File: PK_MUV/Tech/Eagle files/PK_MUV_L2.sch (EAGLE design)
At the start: 6 parts, among them U1 WS2812, U2 WS2812

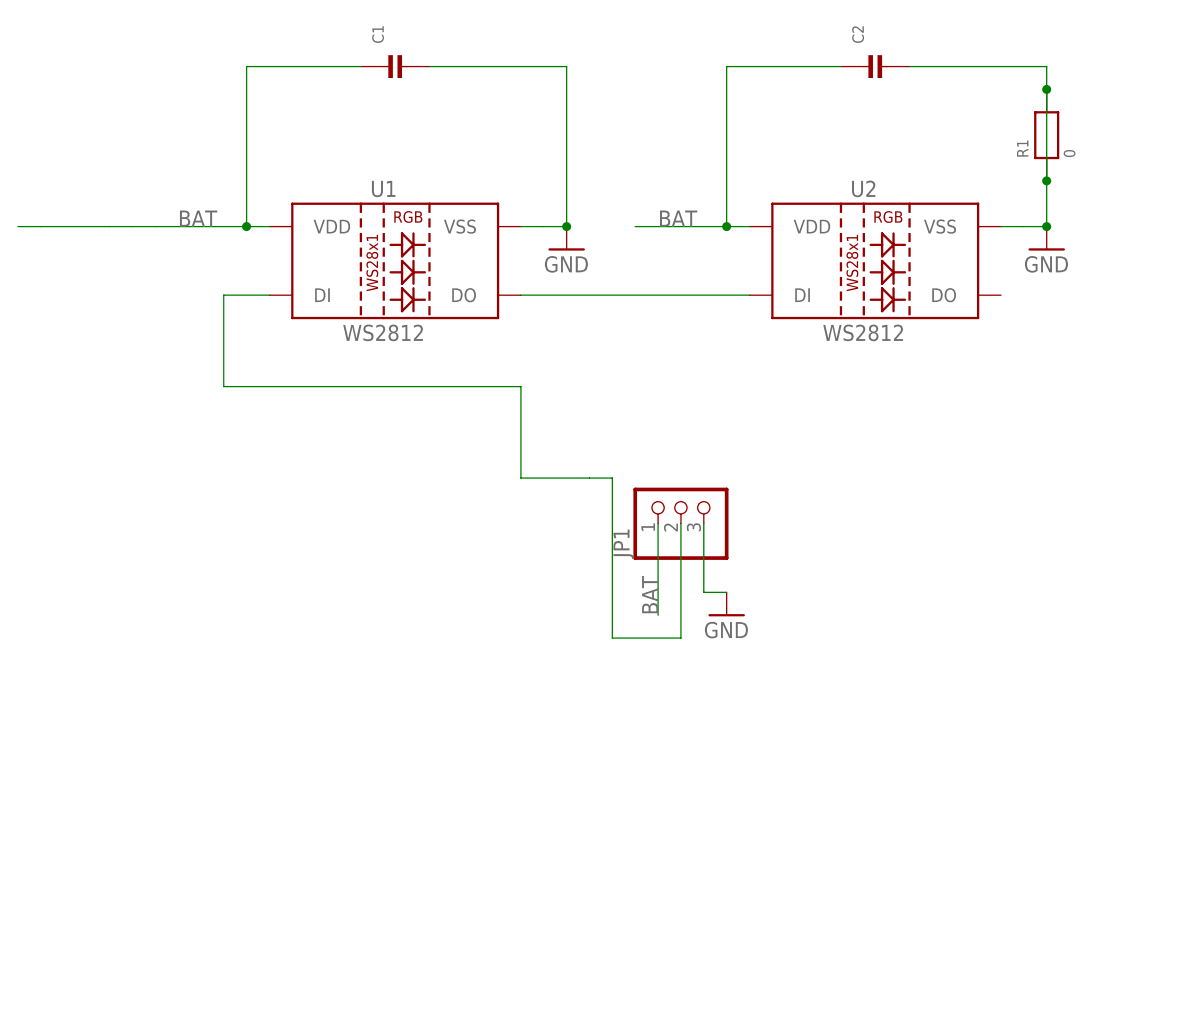
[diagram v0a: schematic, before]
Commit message: Update tech
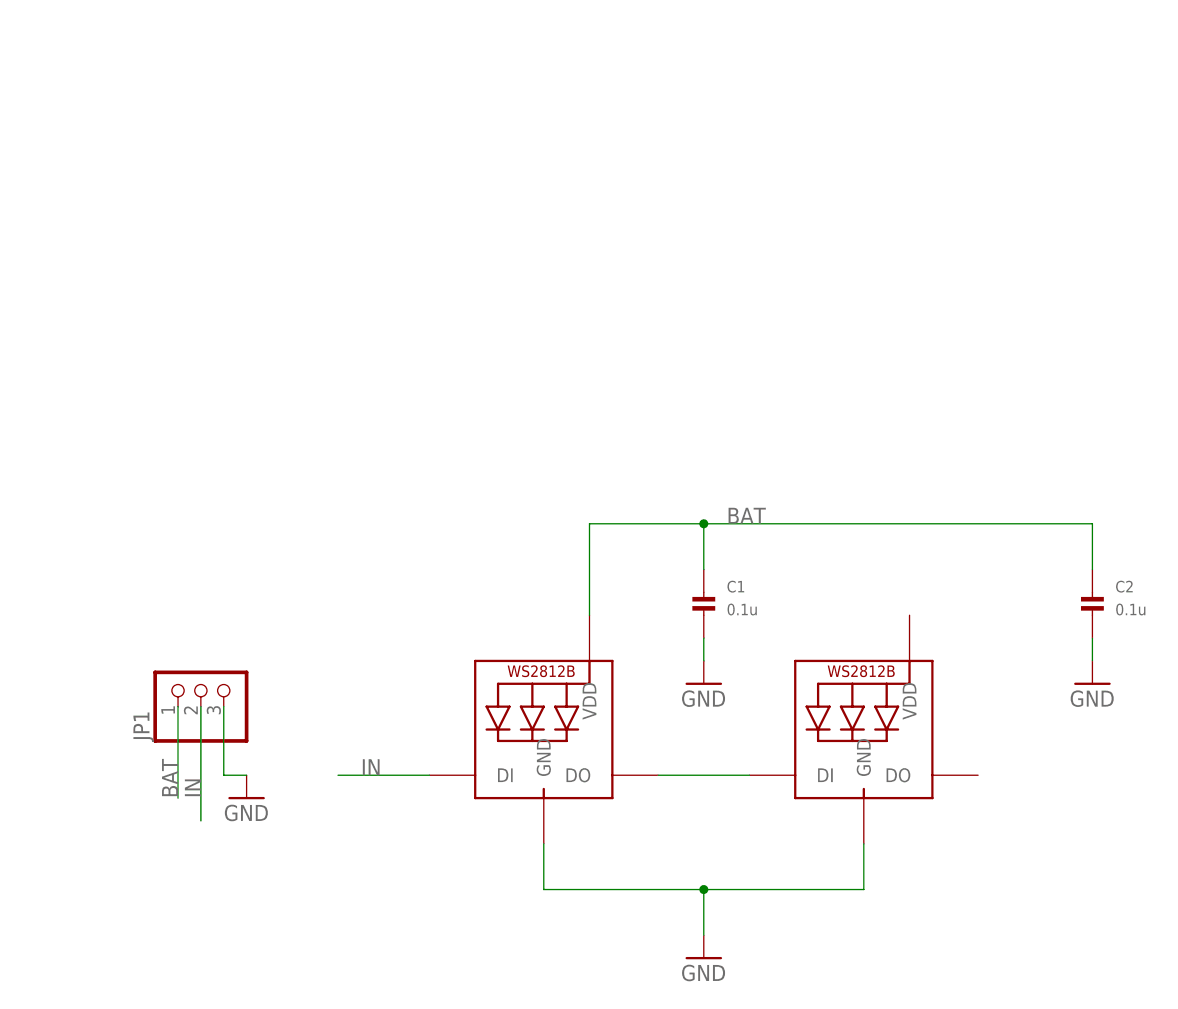
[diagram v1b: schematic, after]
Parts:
- removed R1: 0, microbuilder:RESISTOR1206
- removed U1, U2: WS2812, SparkFun-LED:WS2812"
- added LED1, LED2: WS2812B_5050N, adafruit:WS2812B_5050N
- C1, C2: value (none) -> 0.1u
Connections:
- removed net N$1: JP1.2, U1.DI
- removed net N$2: U1.DO, U2.DI
- new net IN: JP1.2, LED1.DI
- new net N$3: LED1.DO, LED2.DI
- net BAT: now also LED1.VDD; no longer U1.VDD, U2.VDD
- net GND: now also LED1.GND, LED2.GND; no longer R1.1, R1.2, U1.VSS, U2.VSS
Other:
- moved on the sheet: C1, C2, JP1
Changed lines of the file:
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@@
 </classes>
 <parts>
-<part name="U1" library="SparkFun-LED" deviceset="WS2812" device="&quot;" value="WS2812"/>
-<part name="GND2" library="supply1" library_urn="urn:adsk.eagle:library:371" deviceset="GND" device=""/>
-<part name="C1" library="microbuilder" deviceset="CAP_CERAMIC" device="1206"/>
-<part name="U2" library="SparkFun-LED" deviceset="WS2812" device="&quot;" value="WS2812"/>
-<part name="GND3" library="supply1" library_urn="urn:adsk.eagle:library:371" deviceset="GND" device=""/>
-<part name="C2" library="microbuilder" deviceset="CAP_CERAMIC" device="1206"/>
-<part name="R1" library="microbuilder" deviceset="RESISTOR" device="1206" value="0"/>
+<part name="C1" library="microbuilder" deviceset="CAP_CERAMIC" device="1206" value="0.1u"/>
+<part name="C2" library="microbuilder" deviceset="CAP_CERAMIC" device="1206" value="0.1u"/>
 <part name="JP1" library="microbuilder" deviceset="HEADER-1X3" device=""/>
 <part name="GND4" library="supply1" library_urn="urn:adsk.eagle:library:371" deviceset="GND" device=""/>
+<part name="LED1" library="adafruit" deviceset="WS2812B" device="_5050N"/>
+<part name="LED2" library="adafruit" deviceset="WS2812B" device="_5050N"/>
+<part name="GND1" library="supply1" library_urn="urn:adsk.eagle:library:371" deviceset="GND" device=""/>
+<part name="GND5" library="supply1" library_urn="urn:adsk.eagle:library:371" deviceset="GND" device=""/>
+<part name="GND6" library="supply1" library_urn="urn:adsk.eagle:library:371" deviceset="GND" device=""/>
 </parts>
 <sheets>
@@
 </plain>
 <instances>
-<instance part="U1" gate="U1" x="40.64" y="83.82"/>
-<instance part="GND2" gate="1" x="58.42" y="86.36"/>
-<instance part="C1" gate="G$1" x="40.64" y="106.68" rot="R90"/>
-<instance part="U2" gate="U1" x="93.98" y="83.82"/>
-<instance part="GND3" gate="1" x="111.76" y="86.36"/>
-<instance part="C2" gate="G$1" x="93.98" y="106.68" rot="R90"/>
-<instance part="R1" gate="G$1" x="111.76" y="99.06" rot="R90"/>
-<instance part="JP1" gate="A" x="71.12" y="58.42" rot="R90"/>
-<instance part="GND4" gate="1" x="76.2" y="45.72"/>
+<instance part="C1" gate="G$1" x="73.66" y="45.72"/>
+<instance part="C2" gate="G$1" x="116.84" y="45.72"/>
+<instance part="JP1" gate="A" x="17.78" y="38.1" rot="R90"/>
+<instance part="GND4" gate="1" x="22.86" y="25.4"/>
+<instance part="LED1" gate="G$1" x="55.88" y="30.48"/>
+<instance part="LED2" gate="G$1" x="91.44" y="30.48"/>
+<instance part="GND1" gate="1" x="73.66" y="7.62"/>
+<instance part="GND5" gate="1" x="116.84" y="38.1"/>
+<instance part="GND6" gate="1" x="73.66" y="38.1"/>
 </instances>
 <busses>
@@
 <net name="BAT" class="1">
 <segment>
-<pinref part="U1" gate="U1" pin="VDD"/>
-<wire x1="25.4" y1="88.9" x2="22.86" y2="88.9" width="0.1524" layer="91"/>
-<label x="15.24" y="88.9" size="1.778" layer="95"/>
-<pinref part="C1" gate="G$1" pin="P$1"/>
-<wire x1="22.86" y1="88.9" x2="12.7" y2="88.9" width="0.1524" layer="91"/>
-<wire x1="35.56" y1="106.68" x2="22.86" y2="106.68" width="0.1524" layer="91"/>
-<wire x1="22.86" y1="106.68" x2="22.86" y2="88.9" width="0.1524" layer="91"/>
-<junction x="22.86" y="88.9"/>
-<wire x1="12.7" y1="88.9" x2="10.16" y2="88.9" width="0.1524" layer="91"/>
-<wire x1="10.16" y1="88.9" x2="7.62" y2="88.9" width="0.1524" layer="91"/>
-<wire x1="-2.54" y1="88.9" x2="0" y2="88.9" width="0.1524" layer="91"/>
-<wire x1="0" y1="88.9" x2="7.62" y2="88.9" width="0.1524" layer="91"/>
+<pinref part="JP1" gate="A" pin="1"/>
+<wire x1="15.24" y1="35.56" x2="15.24" y2="25.4" width="0.1524" layer="91"/>
+<label x="15.24" y="25.4" size="1.778" layer="95" rot="R90"/>
 </segment>
 <segment>
-<pinref part="U2" gate="U1" pin="VDD"/>
-<wire x1="78.74" y1="88.9" x2="76.2" y2="88.9" width="0.1524" layer="91"/>
+<pinref part="LED1" gate="G$1" pin="VDD"/>
+<wire x1="60.96" y1="45.72" x2="60.96" y2="55.88" width="0.1524" layer="91"/>
+<wire x1="60.96" y1="55.88" x2="73.66" y2="55.88" width="0.1524" layer="91"/>
+<wire x1="73.66" y1="55.88" x2="116.84" y2="55.88" width="0.1524" layer="91"/>
+<wire x1="116.84" y1="55.88" x2="116.84" y2="50.8" width="0.1524" layer="91"/>
+<wire x1="73.66" y1="50.8" x2="73.66" y2="55.88" width="0.1524" layer="91"/>
+<junction x="73.66" y="55.88"/>
 <pinref part="C2" gate="G$1" pin="P$1"/>
-<wire x1="76.2" y1="88.9" x2="66.04" y2="88.9" width="0.1524" layer="91"/>
-<wire x1="88.9" y1="106.68" x2="76.2" y2="106.68" width="0.1524" layer="91"/>
-<wire x1="76.2" y1="106.68" x2="76.2" y2="88.9" width="0.1524" layer="91"/>
-<junction x="76.2" y="88.9"/>
-<label x="68.58" y="88.9" size="1.778" layer="95"/>
-</segment>
-<segment>
-<pinref part="JP1" gate="A" pin="1"/>
-<wire x1="68.58" y1="55.88" x2="68.58" y2="45.72" width="0.1524" layer="91"/>
-<label x="68.58" y="45.72" size="1.778" layer="95" rot="R90"/>
+<pinref part="C1" gate="G$1" pin="P$1"/>
+<label x="76.2" y="55.88" size="1.778" layer="95"/>
 </segment>
 </net>
 <net name="GND" class="1">
 <segment>
-<pinref part="U1" gate="U1" pin="VSS"/>
-<wire x1="53.34" y1="88.9" x2="55.88" y2="88.9" width="0.1524" layer="91"/>
-<pinref part="GND2" gate="1" pin="GND"/>
-<wire x1="55.88" y1="88.9" x2="58.42" y2="88.9" width="0.1524" layer="91"/>
-<pinref part="C1" gate="G$1" pin="P$2"/>
-<wire x1="43.18" y1="106.68" x2="58.42" y2="106.68" width="0.1524" layer="91"/>
-<wire x1="58.42" y1="106.68" x2="58.42" y2="88.9" width="0.1524" layer="91"/>
-<junction x="58.42" y="88.9"/>
+<pinref part="JP1" gate="A" pin="3"/>
+<pinref part="GND4" gate="1" pin="GND"/>
+<wire x1="20.32" y1="35.56" x2="20.32" y2="27.94" width="0.1524" layer="91"/>
+<wire x1="20.32" y1="27.94" x2="22.86" y2="27.94" width="0.1524" layer="91"/>
 </segment>
 <segment>
-<pinref part="U2" gate="U1" pin="VSS"/>
-<wire x1="106.68" y1="88.9" x2="109.22" y2="88.9" width="0.1524" layer="91"/>
-<pinref part="GND3" gate="1" pin="GND"/>
-<wire x1="109.22" y1="88.9" x2="111.76" y2="88.9" width="0.1524" layer="91"/>
-<pinref part="C2" gate="G$1" pin="P$2"/>
-<wire x1="96.52" y1="106.68" x2="111.76" y2="106.68" width="0.1524" layer="91"/>
-<wire x1="111.76" y1="106.68" x2="111.76" y2="104.14" width="0.1524" layer="91"/>
-<junction x="111.76" y="88.9"/>
-<pinref part="R1" gate="G$1" pin="1"/>
-<wire x1="111.76" y1="104.14" x2="111.76" y2="93.98" width="0.1524" layer="91"/>
-<wire x1="111.76" y1="93.98" x2="111.76" y2="88.9" width="0.1524" layer="91"/>
-<junction x="111.76" y="93.98"/>
-<pinref part="R1" gate="G$1" pin="2"/>
-<junction x="111.76" y="104.14"/>
+<pinref part="LED1" gate="G$1" pin="GND"/>
+<wire x1="55.88" y1="20.32" x2="55.88" y2="15.24" width="0.1524" layer="91"/>
+<pinref part="LED2" gate="G$1" pin="GND"/>
+<wire x1="55.88" y1="15.24" x2="73.66" y2="15.24" width="0.1524" layer="91"/>
+<wire x1="73.66" y1="15.24" x2="91.44" y2="15.24" width="0.1524" layer="91"/>
+<wire x1="91.44" y1="15.24" x2="91.44" y2="20.32" width="0.1524" layer="91"/>
+<pinref part="GND1" gate="1" pin="GND"/>
+<wire x1="73.66" y1="10.16" x2="73.66" y2="15.24" width="0.1524" layer="91"/>
+<junction x="73.66" y="15.24"/>
 </segment>
 <segment>
-<pinref part="JP1" gate="A" pin="3"/>
-<pinref part="GND4" gate="1" pin="GND"/>
-<wire x1="73.66" y1="55.88" x2="73.66" y2="48.26" width="0.1524" layer="91"/>
-<wire x1="73.66" y1="48.26" x2="76.2" y2="48.26" width="0.1524" layer="91"/>
+<pinref part="GND5" gate="1" pin="GND"/>
+<wire x1="116.84" y1="43.18" x2="116.84" y2="40.64" width="0.1524" layer="91"/>
+<pinref part="C2" gate="G$1" pin="P$2"/>
+</segment>
+<segment>
+<pinref part="GND6" gate="1" pin="GND"/>
+<wire x1="73.66" y1="43.18" x2="73.66" y2="40.64" width="0.1524" layer="91"/>
+<pinref part="C1" gate="G$1" pin="P$2"/>
 </segment>
 </net>
-<net name="N$1" class="0">
+<net name="IN" class="0">
 <segment>
-<wire x1="53.34" y1="60.96" x2="53.34" y2="71.12" width="0.1524" layer="91"/>
-<wire x1="53.34" y1="71.12" x2="20.32" y2="71.12" width="0.1524" layer="91"/>
-<pinref part="U1" gate="U1" pin="DI"/>
-<wire x1="20.32" y1="71.12" x2="20.32" y2="81.28" width="0.1524" layer="91"/>
-<wire x1="20.32" y1="81.28" x2="25.4" y2="81.28" width="0.1524" layer="91"/>
-<wire x1="53.34" y1="60.96" x2="60.96" y2="60.96" width="0.1524" layer="91"/>
-<wire x1="60.96" y1="60.96" x2="63.5" y2="60.96" width="0.1524" layer="91"/>
-<wire x1="63.5" y1="60.96" x2="63.5" y2="43.18" width="0.1524" layer="91"/>
-<wire x1="63.5" y1="43.18" x2="71.12" y2="43.18" width="0.1524" layer="91"/>
 <pinref part="JP1" gate="A" pin="2"/>
-<wire x1="71.12" y1="43.18" x2="71.12" y2="55.88" width="0.1524" layer="91"/>
+<wire x1="17.78" y1="22.86" x2="17.78" y2="35.56" width="0.1524" layer="91"/>
+<label x="17.78" y="25.4" size="1.778" layer="95" rot="R90"/>
+</segment>
+<segment>
+<pinref part="LED1" gate="G$1" pin="DI"/>
+<wire x1="43.18" y1="27.94" x2="33.02" y2="27.94" width="0.1524" layer="91"/>
+<label x="35.56" y="27.94" size="1.778" layer="95"/>
 </segment>
 </net>
-<net name="N$2" class="0">
+<net name="N$3" class="0">
 <segment>
-<pinref part="U2" gate="U1" pin="DI"/>
-<pinref part="U1" gate="U1" pin="DO"/>
-<wire x1="78.74" y1="81.28" x2="53.34" y2="81.28" width="0.1524" layer="91"/>
+<pinref part="LED1" gate="G$1" pin="DO"/>
+<pinref part="LED2" gate="G$1" pin="DI"/>
+<wire x1="68.58" y1="27.94" x2="78.74" y2="27.94" width="0.1524" layer="91"/>
 </segment>
 </net>
